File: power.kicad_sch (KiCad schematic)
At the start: 60 parts, among them J13 Battery, Q1 AP2302B, SW1 Power, U11 AP3032KTR, U12 AP3032KTR, U15 LR8341A-M25, U23 TPS63020DSJR, U25 65K5., U6 BQ25895RTW

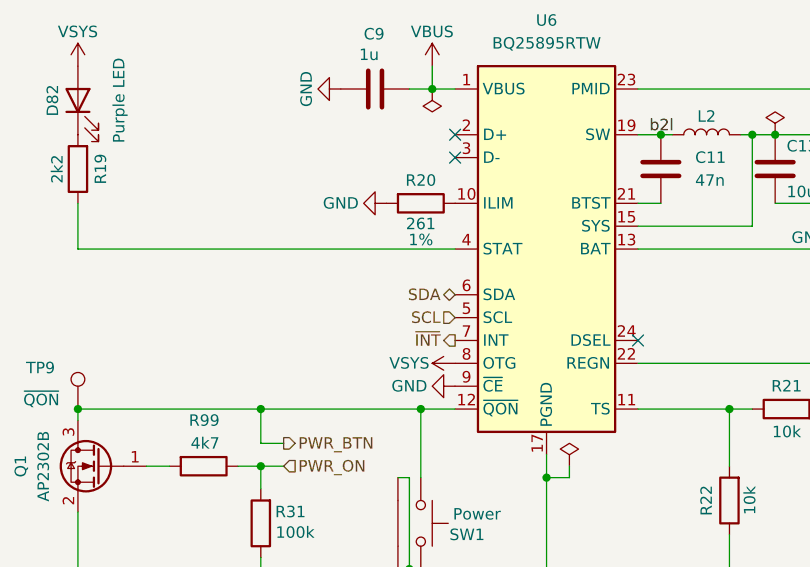
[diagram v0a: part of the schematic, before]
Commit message: Add PCB probe/jumper is i2c bus to PMIC, add Ranzbak logo.
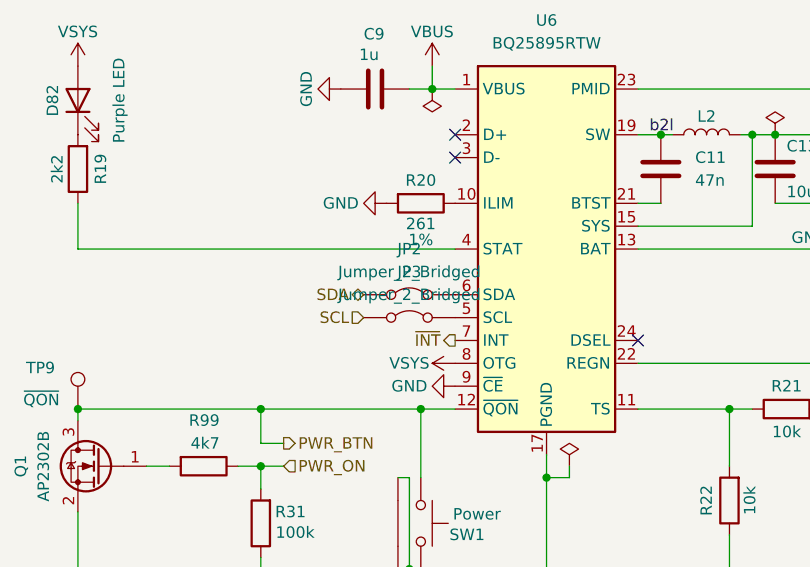
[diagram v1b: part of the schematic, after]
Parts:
- added JP2, JP3: Jumper_2_Bridged, Jumper:SolderJumper-2_P1.3mm_Bridged_RoundedPad1.0x1.5mm, symbol Jumper:Jumper_2_Bridged
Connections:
- net SCL: now also JP3.1 (A); no longer U6.5 (SCL)
- net SDA: now also JP2.1 (A); no longer U6.6 (SDA)
- new net: JP3.2 (B), U6.5 (SCL)
- new net: JP2.2 (B), U6.6 (SDA)
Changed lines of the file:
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@@
 	(hierarchical_label "SCL"
 		(shape input)
-		(at 62.23 57.15 180)
+		(at 52.07 57.15 180)
 		(fields_autoplaced yes)
 		(effects
@@
 	(hierarchical_label "SDA"
 		(shape bidirectional)
-		(at 62.23 54.61 180)
+		(at 52.07 54.61 180)
 		(fields_autoplaced yes)
 		(effects
@@
 	)
 	(symbol
+		(lib_id "Jumper:Jumper_2_Bridged")
+		(at 57.15 54.61 0)
+		(unit 1)
+		(exclude_from_sim yes)
+		(in_bom yes)
+		(on_board yes)
+		(dnp no)
+		(fields_autoplaced yes)
+		(property "Reference" "JP2"
+			(at 57.15 49.53 0)
+			(effects
+				(font
+					(size 1.27 1.27)
+				)
+			)
+		)
+		(property "Value" "Jumper_2_Bridged"
+			(at 57.15 52.07 0)
+			(effects
+				(font
+					(size 1.27 1.27)
+				)
+			)
+		)
+		(property "Footprint" "Jumper:SolderJumper-2_P1.3mm_Bridged_RoundedPad1.0x1.5mm"
+			(at 57.15 54.61 0)
+			(effects
+				(font
+					(size 1.27 1.27)
+				)
+				(hide yes)
+			)
+		)
+		(property "Datasheet" "~"
+			(at 57.15 54.61 0)
+			(effects
+				(font
+					(size 1.27 1.27)
+				)
+				(hide yes)
+			)
+		)
+		(property "Description" "Jumper, 2-pole, closed/bridged"
+			(at 57.15 54.61 0)
+			(effects
+				(font
+					(size 1.27 1.27)
+				)
+				(hide yes)
+			)
+		)
+		(pin "2"
+		)
+		(pin "1"
+		)
+		(instances
+			(project ""
+				(path "/6a31734e-65de-48f3-8156-2b24b665b183/1b21cacd-3ed4-4137-bf19-1f15d3ffa268"
+					(reference "JP2")
+					(unit 1)
+				)
+			)
+		)
+	)
+	(symbol
 		(lib_id "Device:C")
 		(at 234.95 30.48 0)
@@
 					(unit 1)
 				)
+			)
+		)
+	)
+	(symbol
+		(lib_id "Jumper:Jumper_2_Bridged")
+		(at 57.15 57.15 0)
+		(unit 1)
+		(exclude_from_sim yes)
+		(in_bom yes)
+		(on_board yes)
+		(dnp no)
+		(fields_autoplaced yes)
+		(property "Reference" "JP3"
+			(at 57.15 52.07 0)
+			(effects
+				(font
+					(size 1.27 1.27)
+				)
+			)
+		)
+		(property "Value" "Jumper_2_Bridged"
+			(at 57.15 54.61 0)
+			(effects
+				(font
+					(size 1.27 1.27)
+				)
+			)
+		)
+		(property "Footprint" "Jumper:SolderJumper-2_P1.3mm_Bridged_RoundedPad1.0x1.5mm"
+			(at 57.15 57.15 0)
+			(effects
+				(font
+					(size 1.27 1.27)
+				)
+				(hide yes)
+			)
+		)
+		(property "Datasheet" "~"
+			(at 57.15 57.15 0)
+			(effects
+				(font
+					(size 1.27 1.27)
+				)
+				(hide yes)
+			)
+		)
+		(property "Description" "Jumper, 2-pole, closed/bridged"
+			(at 57.15 57.15 0)
+			(effects
+				(font
+					(size 1.27 1.27)
+				)
+				(hide yes)
+			)
+		)
+		(pin "2"
+		)
+		(pin "1"
+		)
+		(instances
+			(project "why2025"
+				(path "/6a31734e-65de-48f3-8156-2b24b665b183/1b21cacd-3ed4-4137-bf19-1f15d3ffa268"
+					(reference "JP3")
+					(unit 1)
+				)

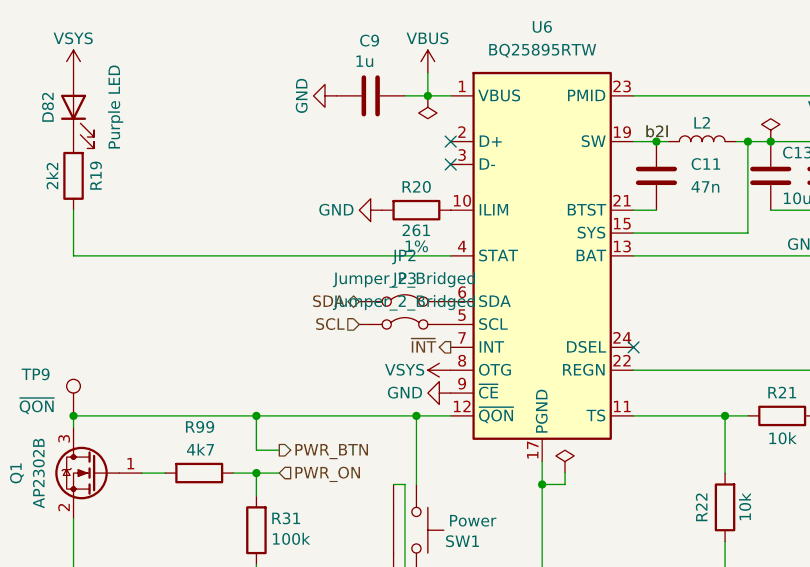
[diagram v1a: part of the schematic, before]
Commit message: Add Bosch logo, first attempt at creating thermal separation for BME690
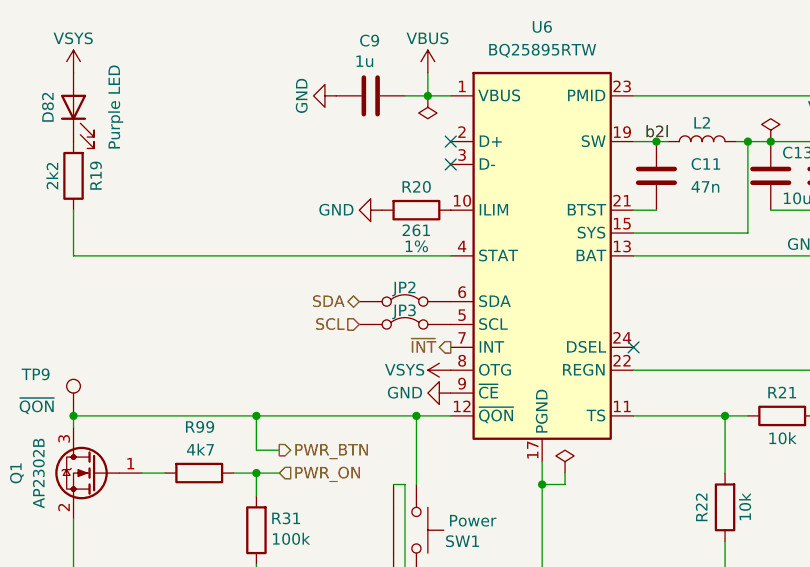
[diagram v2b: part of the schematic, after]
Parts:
- JP2, JP3: value Jumper_2_Bridged -> (none); now left out of the parts list
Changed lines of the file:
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@@
 		(unit 1)
 		(exclude_from_sim yes)
-		(in_bom yes)
+		(in_bom no)
 		(on_board yes)
 		(dnp no)
-		(fields_autoplaced yes)
 		(property "Reference" "JP2"
-			(at 57.15 49.53 0)
+			(at 57.15 53.086 0)
 			(effects
 				(font
@@
 			)
 		)
-		(property "Value" "Jumper_2_Bridged"
+		(property "Value" ""
 			(at 57.15 52.07 0)
 			(effects
@@
 			)
 		)
-		(property "Datasheet" "~"
+		(property "Datasheet" ""
 			(at 57.15 54.61 0)
 			(effects
@@
 			)
 		)
-		(property "Description" "Jumper, 2-pole, closed/bridged"
+		(property "Description" ""
 			(at 57.15 54.61 0)
 			(effects
@@
 		(unit 1)
 		(exclude_from_sim yes)
-		(in_bom yes)
+		(in_bom no)
 		(on_board yes)
 		(dnp no)
-		(fields_autoplaced yes)
 		(property "Reference" "JP3"
-			(at 57.15 52.07 0)
+			(at 57.15 55.626 0)
 			(effects
 				(font
@@
 			)
 		)
-		(property "Value" "Jumper_2_Bridged"
+		(property "Value" ""
 			(at 57.15 54.61 0)
 			(effects
@@
 			)
 		)
-		(property "Datasheet" "~"
+		(property "Datasheet" ""
 			(at 57.15 57.15 0)
 			(effects
@@
 			)
 		)
-		(property "Description" "Jumper, 2-pole, closed/bridged"
+		(property "Description" ""
 			(at 57.15 57.15 0)
 			(effects

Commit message: Add LCSC number for ESP32-P4
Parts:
- JP2, JP3: value (none) -> ~
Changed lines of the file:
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@@
 			)
 		)
-		(property "Value" ""
+		(property "Value" "~"
 			(at 57.15 52.07 0)
 			(effects
@@
 			)
 		)
-		(property "Value" ""
+		(property "Value" "~"
 			(at 57.15 54.61 0)
 			(effects
